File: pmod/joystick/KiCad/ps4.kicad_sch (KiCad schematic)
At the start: 5 parts, among them J2 Conn_01x05_Pin, U1 COM-09032

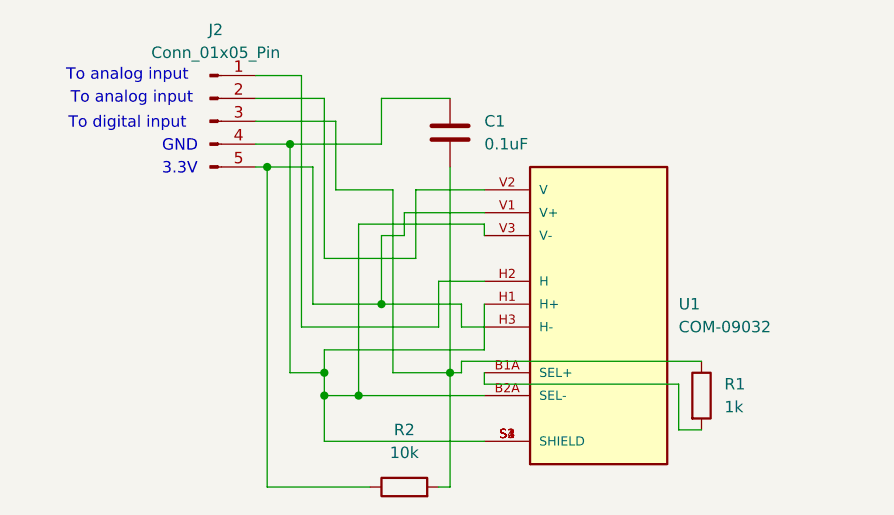
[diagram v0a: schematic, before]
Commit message: better schematic
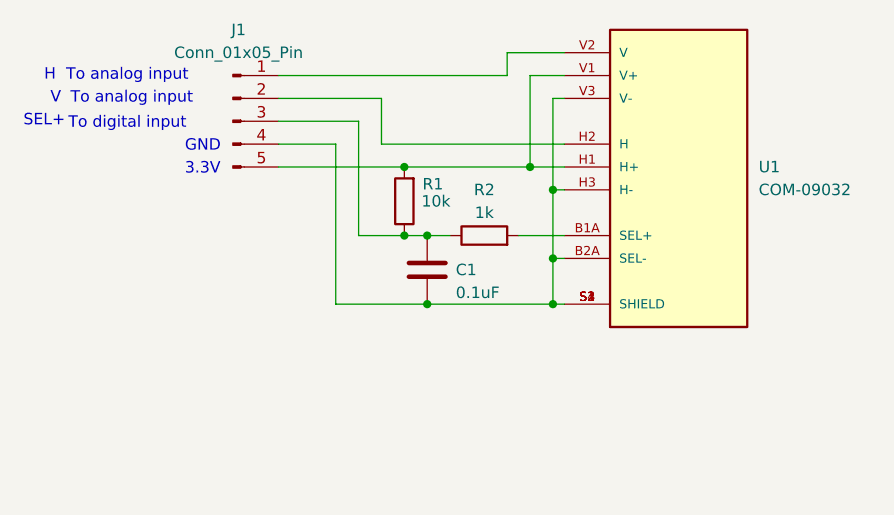
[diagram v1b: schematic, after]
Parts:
- renumbered J2 to J1, R2 to R1, R1 to R2
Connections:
- net at J1.3 (Pin_3), R2.1: now also C1.1, R1.1; no longer C1.2, R1.2
- net at J1.4 (Pin_4), U1.B2A (SEL-), U1.S1 (SHIELD)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: now also C1.2, U1.H3 (H-); no longer C1.1, U1.H1 (H+)
- net at U1.H2 (H): now also J1.2 (Pin_2); no longer J1.1 (Pin_1)
- net at J1.5 (Pin_5), U1.V1 (V+): now also R1.2, U1.H1 (H+); no longer R1.1, U1.H3 (H-)
- net at U1.V2 (V): now also J1.1 (Pin_1); no longer J1.2 (Pin_2)
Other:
- note added: "H"
- note added: "SEL+"
- note added: "V"
- moved on the sheet: C1, J1, R1, R2, U1
